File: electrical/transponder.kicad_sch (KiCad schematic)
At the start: 4 parts

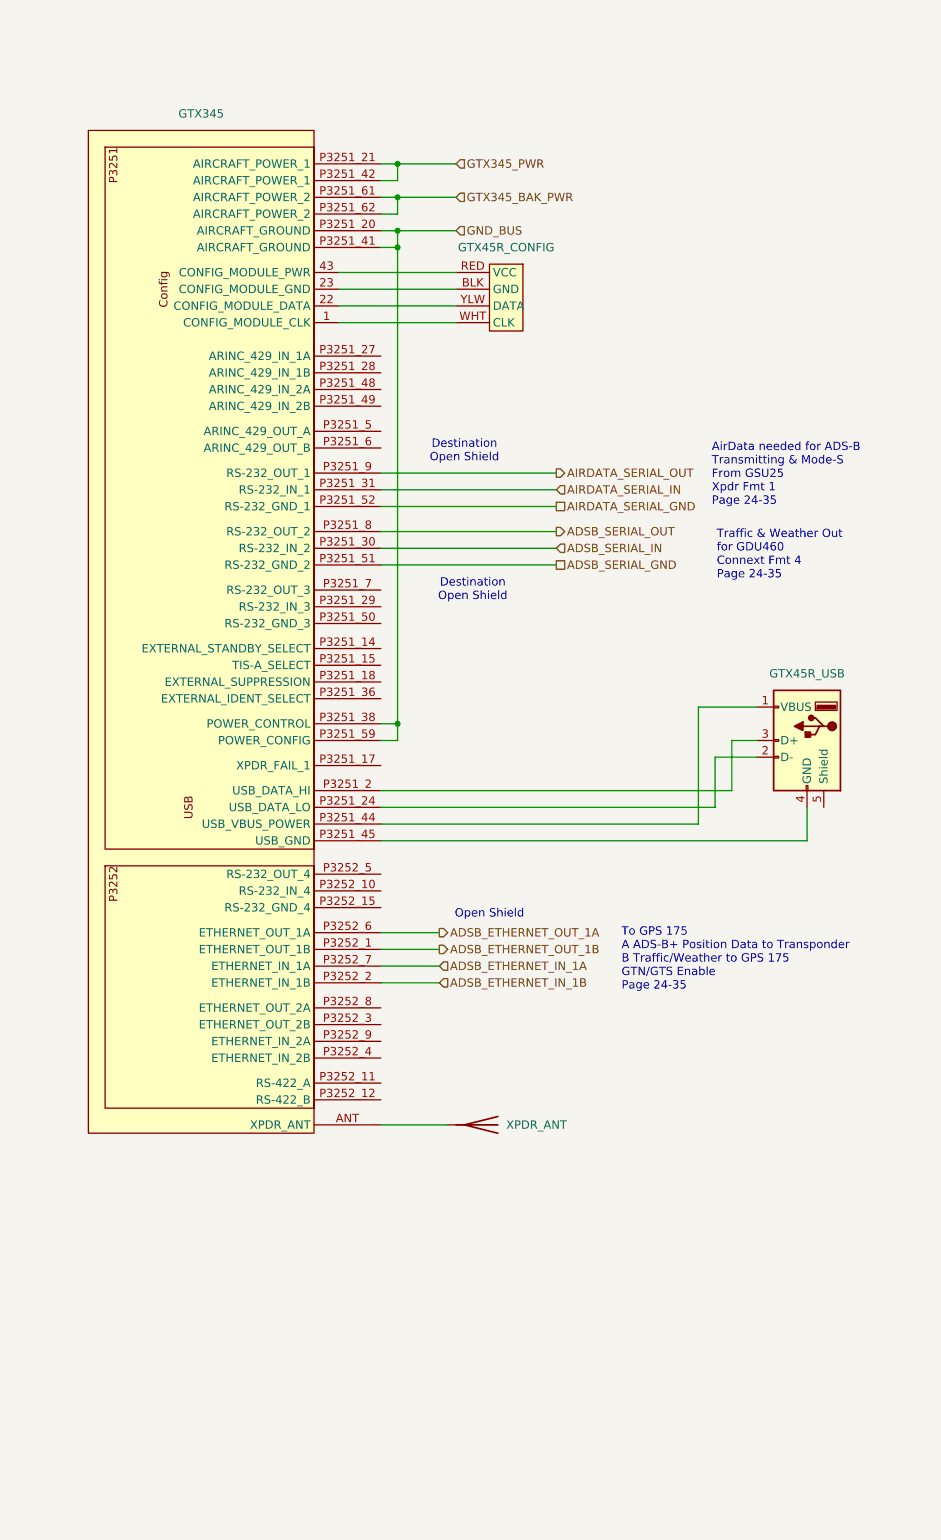
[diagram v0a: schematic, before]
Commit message: Added lighting bus
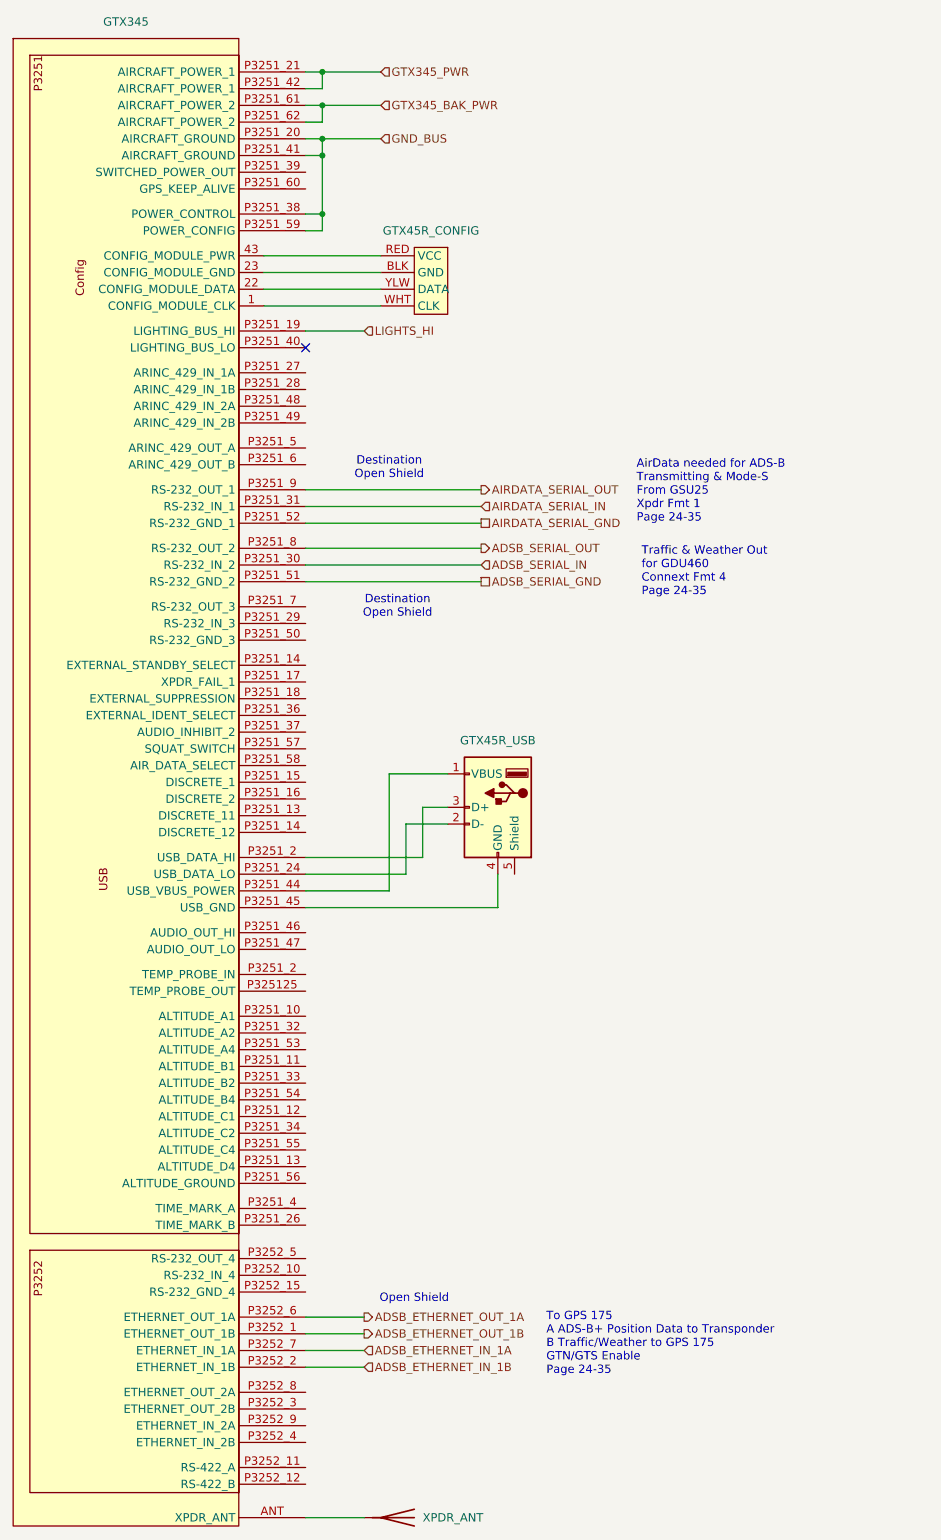
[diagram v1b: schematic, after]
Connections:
- new net LIGHTS_HI: GTX345.P3251_19 (LIGHTING_BUS_HI)
- no-connect marks 0 -> 1
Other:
- moved on the sheet: GTX45R_CONFIG, GTX45R_USB, XPDR_ANT
